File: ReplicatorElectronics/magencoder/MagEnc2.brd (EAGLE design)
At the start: 44.5 x 44.5 mm, 13 parts, among them J1 SBH11-PBPC-D07-ST-BK, J2 70553-0037, T1 MMBT2222A

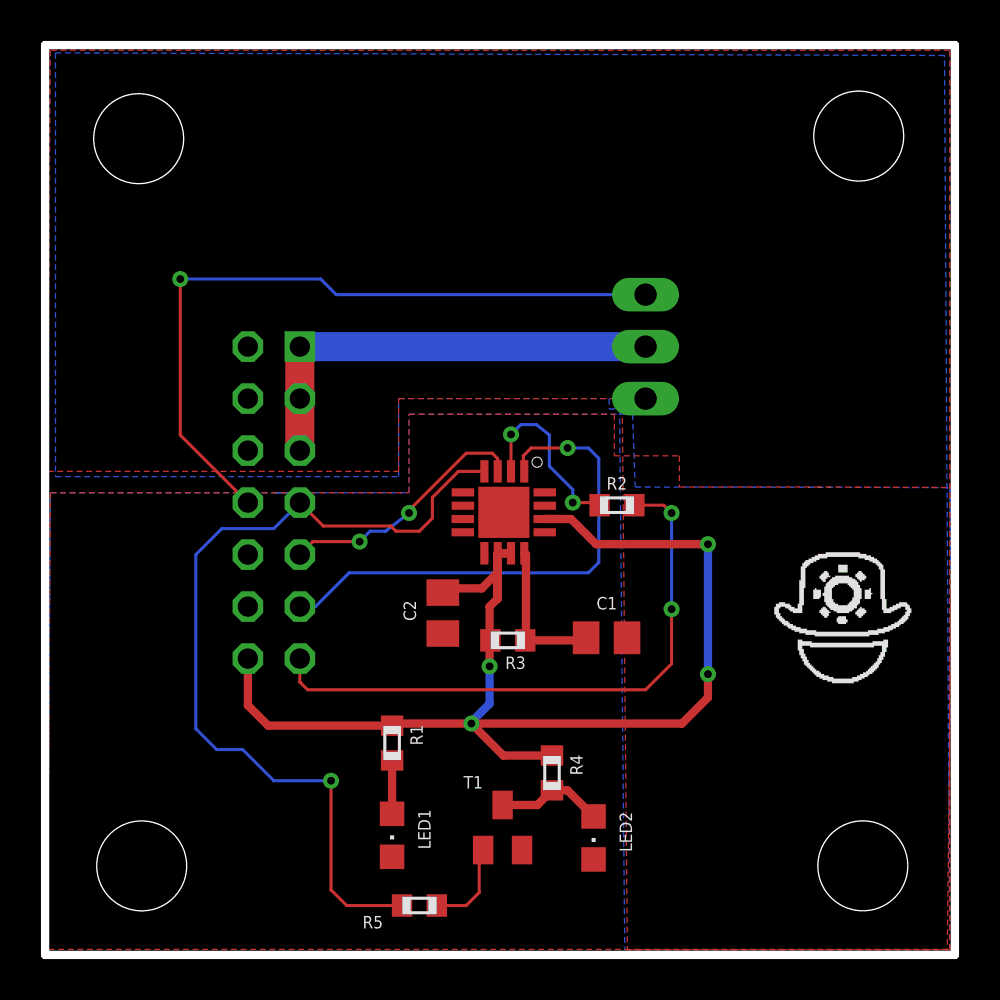
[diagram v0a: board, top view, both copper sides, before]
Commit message: 6/4/12: New, smaller size.
~ 1.5 hrs.
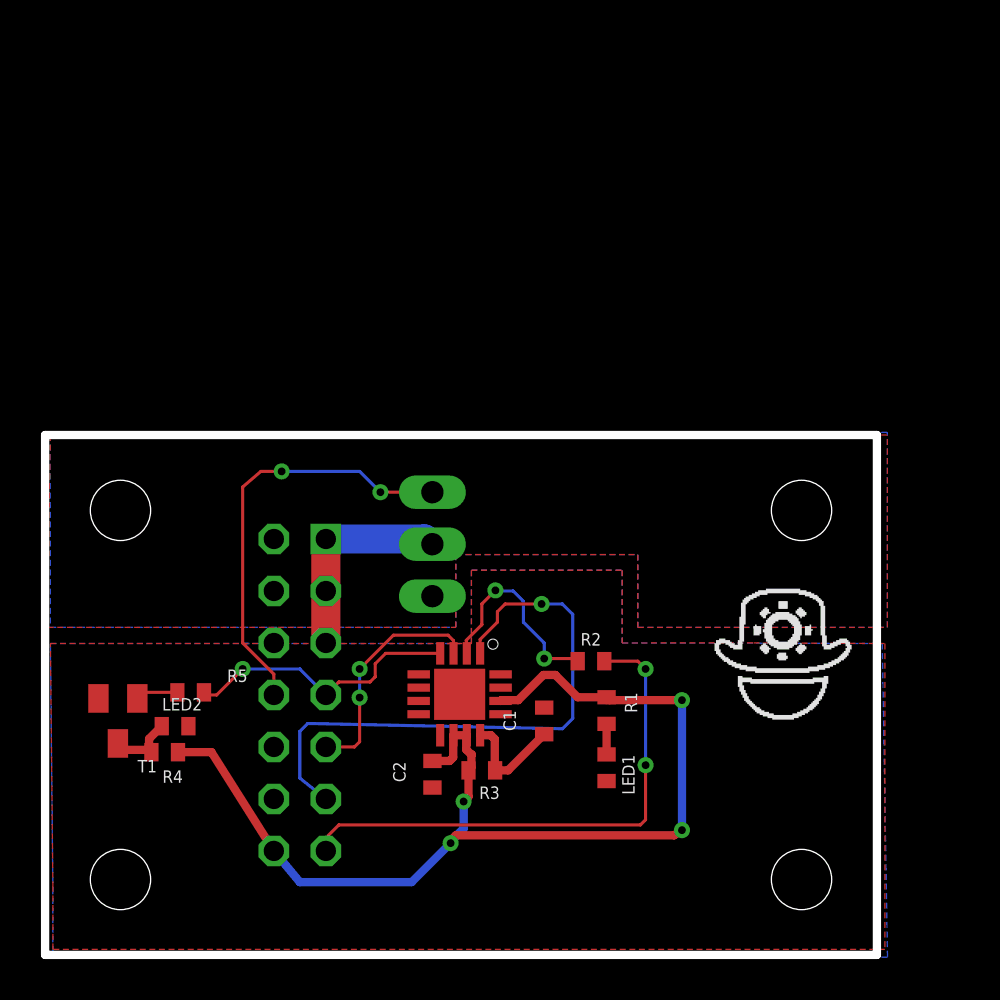
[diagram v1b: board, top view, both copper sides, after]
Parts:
- C1, C2: device rcl:C0805K -> resistor:C0402
- LED1, LED2: device led:CHIPLED_0805 -> resistor:R0402
- R1, R2, R3, R4, R5: device rcl:R0603 -> resistor:R0402
- moved LED2 21.2 mm to (6.35, 11.2), turned to 0 degrees
- moved T1 19.5 mm to (3.56, 11.4), turned to 180 degrees
- moved R4 19.0 mm to (5.84, 9.91), turned to 180 degrees
- moved R5 15.3 mm to (7.11, 12.8), turned to 0 degrees
- moved J2 14.2 mm to (26.5, 20.1)
- moved LED1 11.0 mm to (27.4, 9.14), turned to 270 degrees
- moved R1 10.6 mm to (27.4, 11.9)
- moved J1 9.48 mm to (13.7, 20.3)
- moved U$2 9.15 mm to (19.3, 14.7)
- moved C2 7.89 mm to (18.9, 8.83)
- moved R2 7.73 mm to (26.7, 14.4)
- moved R3 6.48 mm to (21.3, 9.02)
- moved C1 5.08 mm to (24.4, 11.4), turned to 90 degrees
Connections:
- net DGND: now also LED1.2, LED2.2; no longer LED1.C, LED2.C
- net N$1: now also LED1.1; no longer LED1.A
- net N$2: now also LED2.1; no longer LED2.A
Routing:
- net CSN: track 42.8 -> 13.9 mm
- net SERVO_CTRL: track 35.3 -> 20.8 mm, vias 1 -> 2
- net 5V_SERVO: track 22.0 -> 10.4 mm
- net VCC: track 62.0 -> 54.2 mm
- net MOSI: track 25.4 -> 29.1 mm
- net MISO: track 29.3 -> 26.2 mm
- net N$3: track 4.49 -> 2.08 mm
- net N$2: track 5.27 -> 3.23 mm
- net VDD: track 7.34 -> 5.62 mm
- net SCLK: track 12.5 -> 11.3 mm
- net N$1: track 2.61 -> 1.49 mm
- net N$4: track 9.10 -> 9.93 mm
- net DGND: track 0.59 -> 0.00 mm
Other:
- board size 44.5 x 44.5 mm -> 40.6 x 25.4 mm
- board text added: "Mounting holes are 4-40 (0.116")"
- board text added: "Rev. 7"
- board text removed: "Mounting holes are 8-32 (0.173")"
- board text removed: "Rev. 6"

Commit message: 6/3/12: Corrections to size reduction.
~ 1 hr.
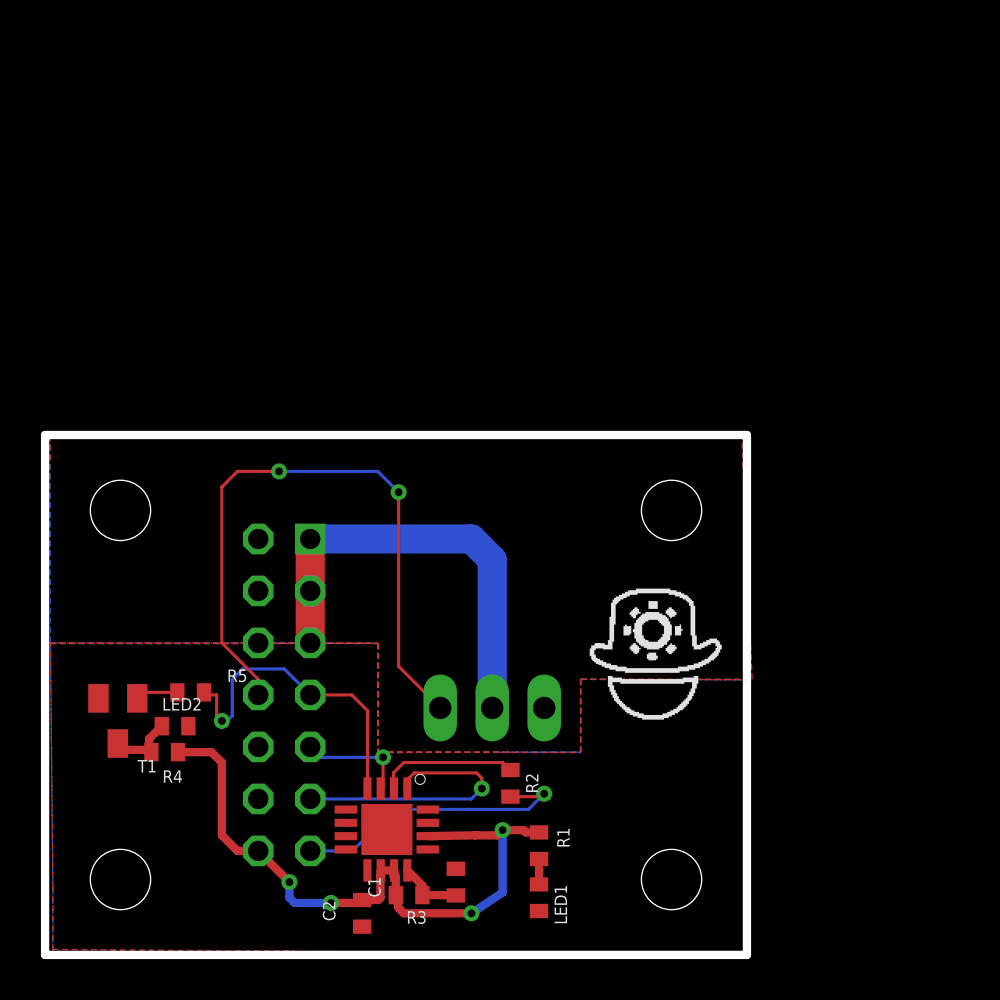
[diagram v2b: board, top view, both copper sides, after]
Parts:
- moved C1 8.98 mm to (20.1, 3.56)
- moved C2 7.61 mm to (15.5, 2.03)
- moved U$2 7.50 mm to (15.7, 8.13)
- moved R1 7.38 mm to (24.1, 5.33)
- moved LED1 7.16 mm to (24.1, 2.79)
- moved R2 7.15 mm to (22.7, 8.38), turned to 270 degrees
- moved R3 7.06 mm to (17.8, 2.92)
- moved J2 4.71 mm to (21.8, 19.7), turned to 0 degrees
- moved J1 0.76 mm to (13.0, 20.3)
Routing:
- net VCC: track 54.2 -> 34.0 mm
- net MOSI: track 29.1 -> 13.4 mm
- net MISO: track 26.2 -> 14.2 mm, vias 2 -> 1
- net 5V_SERVO: track 10.4 -> 21.6 mm
- net SERVO_CTRL: track 20.8 -> 31.7 mm
- net SCLK: track 11.3 -> 5.34 mm, vias 2 -> 1
- net N$4: track 9.93 -> 6.87 mm, vias 2 -> 0
- net VDD: track 5.62 -> 3.15 mm
- net CSN: track 13.9 -> 15.9 mm
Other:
- board size 40.6 x 25.4 mm -> 34.3 x 25.4 mm
